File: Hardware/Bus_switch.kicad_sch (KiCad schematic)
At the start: 15 parts, among them J301 Conn_01x04_Pin, U301 SN74CB3Q3384APW

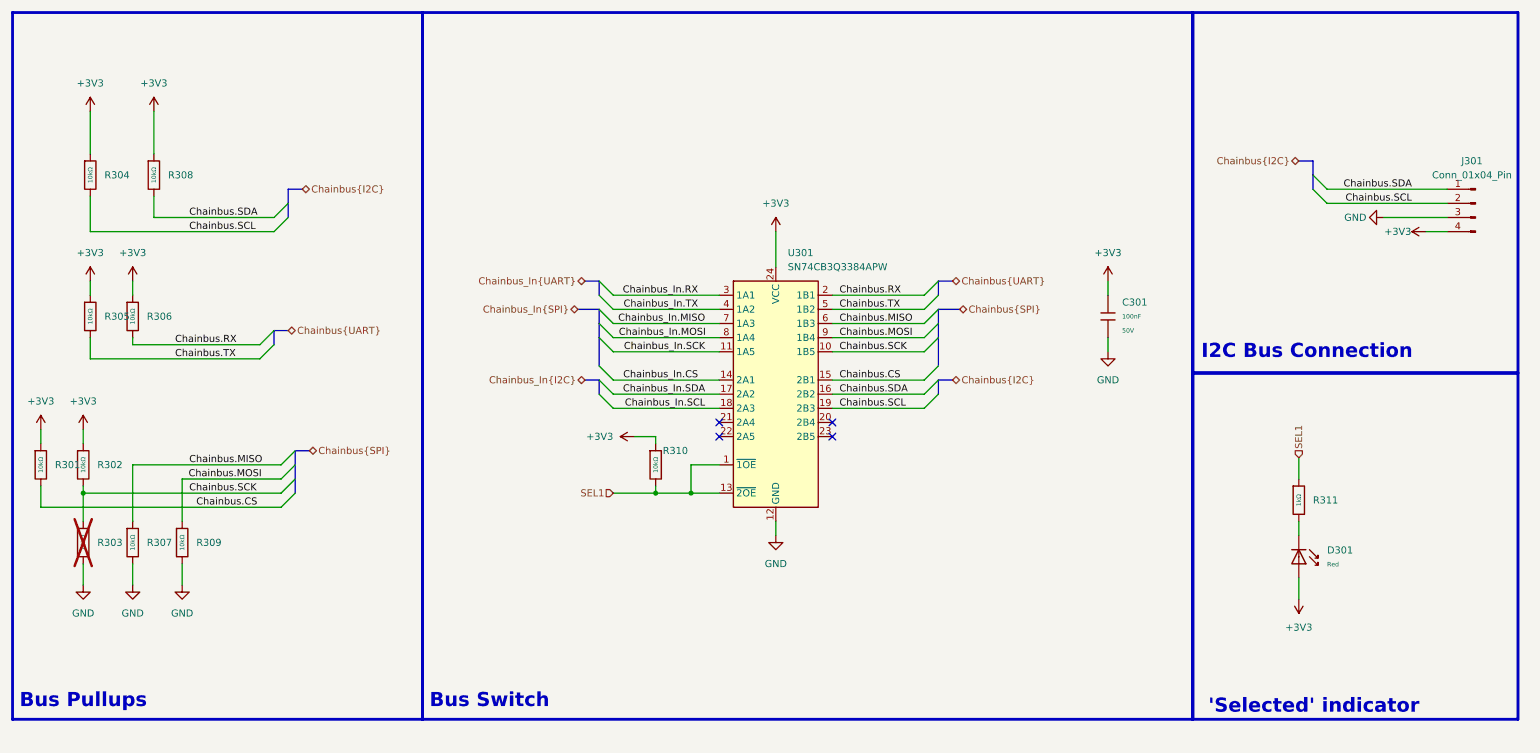
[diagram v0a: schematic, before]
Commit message: major rework of template
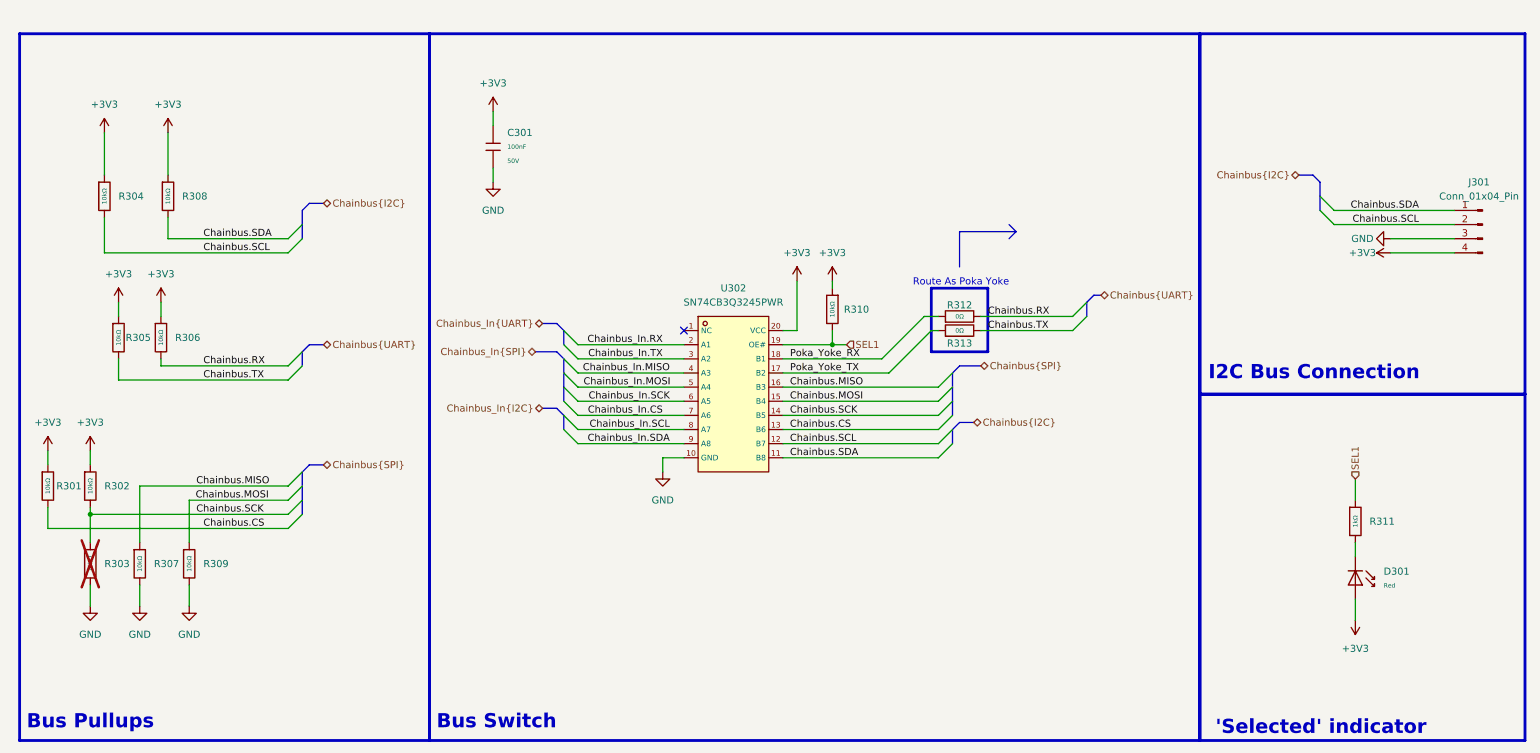
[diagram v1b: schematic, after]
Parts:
- removed U301: SN74CB3Q3384APW, Package_SO:TSSOP-24_4.4x7.8mm_P0.65mm, symbol 74xx:SN74CB3Q3384APW
- added R312, R313: 0Ω, PCM_JLCPCB:R_0603, symbol PCM_JLCPCB-Resistors:0603,0Ω
- added U302: SN74CB3Q3245PWR, lcsc_footprints:C470961_TSSOP-20_L6_5-W4_4-P0_65-LS6_4-BL, symbol Kicad LCSC Manager:SN74CB3Q3245PWR
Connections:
- net +3V3: now also U302.20 (VCC)
- net Chainbus.CS: now also U302.13 (B6)
- net Chainbus.MISO: now also U302.16 (B3)
- net Chainbus.MOSI: now also U302.15 (B4)
- net Chainbus.RX: now also R312.2
- net Chainbus.SCK: now also U302.14 (B5)
- net Chainbus.SCL: now also U302.12 (B7)
- net Chainbus.SDA: now also U302.11 (B8)
- net Chainbus.TX: now also R313.2
- net Chainbus_In.CS: now also U302.7 (A6)
- net Chainbus_In.MISO: now also U302.4 (A3)
- net Chainbus_In.MOSI: now also U302.5 (A4)
- net Chainbus_In.RX: now also U302.2 (A1)
- net Chainbus_In.SCK: now also U302.6 (A5)
- net Chainbus_In.SCL: now also U302.8 (A7)
- net Chainbus_In.SDA: now also U302.9 (A8)
- net Chainbus_In.TX: now also U302.3 (A2)
- net GND: now also U302.10 (GND)
- net SEL1: now also U302.19 (OE#)
- new net Poka_Yoke_RX: R312.1, U302.18 (B1)
- new net Poka_Yoke_TX: R313.1, U302.17 (B2)
- no-connect marks 4 -> 1
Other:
- note added: "Route As Poka Yoke"
